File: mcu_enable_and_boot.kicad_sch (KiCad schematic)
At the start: 12 parts, among them SW1 TS_Basic_Small, SW2 TS_Basic_Small

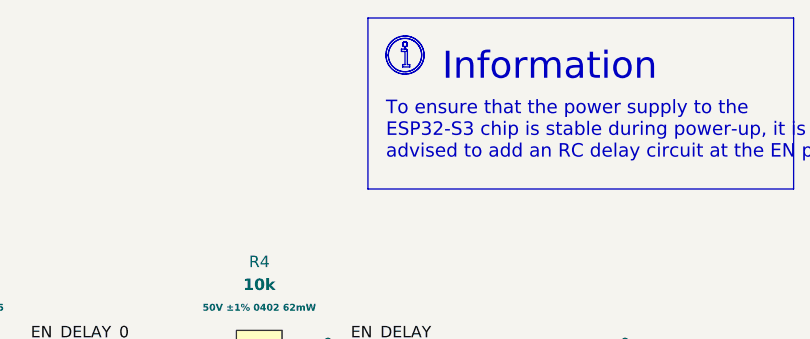
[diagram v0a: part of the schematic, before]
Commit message: Work on kibot
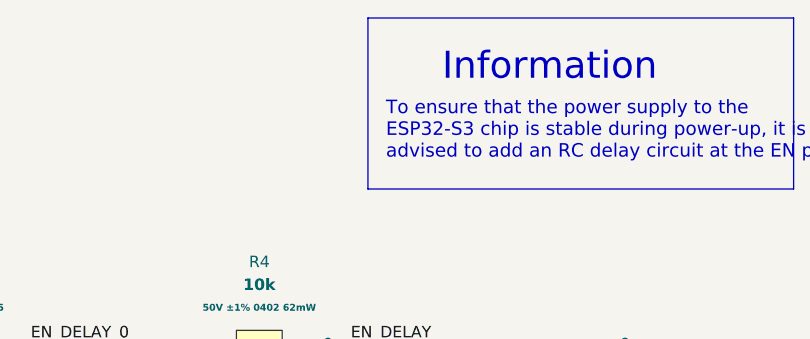
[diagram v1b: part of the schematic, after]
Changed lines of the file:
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@@
-		)
-	)
-	(polyline
-		(pts
-			(xy 127.9603 42.8818) (xy 127.9737 42.8828) (xy 127.987 42.8845) (xy 128 42.8868) (xy 128.0128 42.8898)
-			(xy 128.0253 42.8934) (xy 128.0376 42.8975) (xy 128.0497 42.9023) (xy 128.0614 42.9075) (xy 128.0728 42.9134)
-			(xy 128.0839 42.9198) (xy 128.0946 42.9266) (xy 128.105 42.934) (xy 128.115 42.9419) (xy 128.1246 42.9502)
-			(xy 128.1338 42.959) (xy 128.1425 42.9681) (xy 128.1508 42.9777) (xy 128.1587 42.9877) (xy 128.1661 42.9981)
-			(xy 128.1729 43.0088) (xy 128.1793 43.0199) (xy 128.1852 43.0313) (xy 128.1905 43.0431) (xy 128.1952 43.0551)
-			(xy 128.1994 43.0674) (xy 128.2029 43.0799) (xy 128.2059 43.0927) (xy 128.2082 43.1057) (xy 128.2099 43.119)
-			(xy 128.2109 43.1324) (xy 128.2112 43.146) (xy 128.2109 43.1597) (xy 128.2099 43.1731) (xy 128.2082 43.1863)
-			(xy 128.2059 43.1994) (xy 128.2029 43.2122) (xy 128.1994 43.2247) (xy 128.1952 43.237) (xy 128.1905 43.249)
-			(xy 128.1852 43.2607) (xy 128.1793 43.2722) (xy 128.1729 43.2832) (xy 128.1661 43.294) (xy 128.1587 43.3043)
-			(xy 128.1508 43.3143) (xy 128.1425 43.3239) (xy 128.1338 43.3331) (xy 128.1246 43.3419) (xy 128.115 43.3502)
-			(xy 128.105 43.3581) (xy 128.0946 43.3654) (xy 128.0839 43.3723) (xy 128.0728 43.3787) (xy 128.0614 43.3845)
-			(xy 128.0497 43.3898) (xy 128.0376 43.3946) (xy 128.0253 43.3987) (xy 128.0128 43.4023) (xy 128 43.4052)
-			(xy 127.987 43.4076) (xy 127.9737 43.4093) (xy 127.9603 43.4103) (xy 127.9467 43.4106) (xy 127.9331 43.4103)
-			(xy 127.9196 43.4093) (xy 127.9064 43.4076) (xy 127.8933 43.4052) (xy 127.8805 43.4023) (xy 127.868 43.3987)
-			(xy 127.8557 43.3946) (xy 127.8437 43.3898) (xy 127.832 43.3845) (xy 127.8206 43.3787) (xy 127.8095 43.3723)
-			(xy 127.7987 43.3654) (xy 127.7884 43.3581) (xy 127.7784 43.3502) (xy 127.7688 43.3419) (xy 127.7596 43.3331)
-			(xy 127.7508 43.3239) (xy 127.7425 43.3143) (xy 127.7346 43.3043) (xy 127.7273 43.294) (xy 127.7204 43.2832)
-			(xy 127.714 43.2722) (xy 127.7082 43.2607) (xy 127.7029 43.249) (xy 127.6981 43.237) (xy 127.694 43.2247)
-			(xy 127.6904 43.2122) (xy 127.6875 43.1994) (xy 127.6851 43.1863) (xy 127.6834 43.1731) (xy 127.6824 43.1597)
-			(xy 127.6821 43.146) (xy 127.6824 43.1324) (xy 127.6834 43.119) (xy 127.6851 43.1057) (xy 127.6875 43.0927)
-			(xy 127.6904 43.0799) (xy 127.694 43.0674) (xy 127.6981 43.0551) (xy 127.7029 43.0431) (xy 127.7082 43.0313)
-			(xy 127.714 43.0199) (xy 127.7204 43.0088) (xy 127.7273 42.9981) (xy 127.7346 42.9877) (xy 127.7425 42.9777)
-			(xy 127.7508 42.9681) (xy 127.7596 42.959) (xy 127.7688 42.9502) (xy 127.7784 42.9419) (xy 127.7884 42.934)
-			(xy 127.7987 42.9266) (xy 127.8095 42.9198) (xy 127.8206 42.9134) (xy 127.832 42.9075) (xy 127.8437 42.9023)
-			(xy 127.8557 42.8975) (xy 127.868 42.8934) (xy 127.8805 42.8898) (xy 127.8933 42.8868) (xy 127.9064 42.8845)
-			(xy 127.9196 42.8828) (xy 127.9331 42.8818) (xy 127.9467 42.8815) (xy 127.9603 42.8818)
-		)
-		(stroke
-			(width -0.0001)
-			(type solid)
-		)
-		(fill
-			(type color)
-			(color 34 187 51 1)
-		)
-	)
-	(polyline
-		(pts
-			(xy 127.9598 43.6755) (xy 127.9728 43.6765) (xy 127.9857 43.6781) (xy 127.9985 43.6803) (xy 128.0112 43.6832)
-			(xy 128.0236 43.6866) (xy 128.0359 43.6907) (xy 128.0479 43.6953) (xy 128.0597 43.7006) (xy 128.0713 43.7064)
-			(xy 128.0825 43.7127) (xy 128.0935 43.7197) (xy 128.1041 43.7271) (xy 128.1143 43.7351) (xy 128.1242 43.7437)
-			(xy 128.1338 43.7527) (xy 128.1428 43.7622) (xy 128.1513 43.7721) (xy 128.1593 43.7824) (xy 128.1668 43.793)
-			(xy 128.1737 43.8039) (xy 128.1801 43.8152) (xy 128.1859 43.8267) (xy 128.1911 43.8385) (xy 128.1958 43.8506)
-			(xy 128.1998 43.8628) (xy 128.2033 43.8753) (xy 128.2061 43.8879) (xy 128.2084 43.9007) (xy 128.21 43.9136)
-			(xy 128.2109 43.9267) (xy 128.2112 43.9398) (xy 128.2112 45.395) (xy 128.4758 45.395) (xy 128.4758 45.6596)
-			(xy 127.6821 45.6596) (xy 127.6821 45.395) (xy 127.9467 45.395) (xy 127.9467 43.9398) (xy 127.5498 43.9398)
-			(xy 127.5498 43.6752) (xy 127.9467 43.6752) (xy 127.9598 43.6755)
-		)
-		(stroke
-			(width -0.0001)
-			(type solid)
-		)
-		(fill
-			(type color)
-			(color 34 187 51 1)
 		)
 	)
@@
 		)
 	)
-	(polyline
-		(pts
-			(xy 128.0516 42.2226) (xy 128.1559 42.2304) (xy 128.2592 42.2432) (xy 128.3615 42.261) (xy 128.4626 42.2838)
-			(xy 128.5623 42.3115) (xy 128.6604 42.3439) (xy 128.7567 42.3811) (xy 128.8511 42.4229) (xy 128.9434 42.4694)
-			(xy 129.0334 42.5203) (xy 129.121 42.5756) (xy 129.206 42.6353) (xy 129.2881 42.6993) (xy 129.3673 42.7676)
-			(xy 129.4434 42.84) (xy 129.5158 42.916) (xy 129.584 42.9952) (xy 129.648 43.0774) (xy 129.7077 43.1623)
-			(xy 129.7631 43.2499) (xy 129.814 43.3399) (xy 129.8604 43.4323) (xy 129.9022 43.5267) (xy 129.9394 43.623)
-			(xy 129.9718 43.7211) (xy 129.9995 43.8207) (xy 130.0223 43.9218) (xy 130.0401 44.0241) (xy 130.053 44.1275)
-			(xy 130.0607 44.2317) (xy 130.0633 44.3367) (xy 130.0618 44.4167) (xy 130.0573 44.4961) (xy 130.0499 44.5749)
-			(xy 130.0396 44.6531) (xy 130.0265 44.7304) (xy 130.0105 44.807) (xy 129.9918 44.8826) (xy 129.9704 44.9573)
-			(xy 129.9463 45.031) (xy 129.9196 45.1036) (xy 129.8903 45.175) (xy 129.8584 45.2452) (xy 129.8241 45.3142)
-			(xy 129.7873 45.3818) (xy 129.7482 45.4479) (xy 129.7066 45.5126) (xy 129.6627 45.5758) (xy 129.6166 45.6373)
-			(xy 129.5682 45.6971) (xy 129.5177 45.7552) (xy 129.465 45.8115) (xy 129.4102 45.8659) (xy 129.3534 45.9184)
-			(xy 129.2945 45.9688) (xy 129.2337 46.0172) (xy 129.171 46.0634) (xy 129.1064 46.1075) (xy 129.0399 46.1492)
-			(xy 128.9717 46.1887) (xy 128.9017 46.2257) (xy 128.83 46.2602) (xy 128.7567 46.2922) (xy 128.6071 46.3477)
-			(xy 128.4553 46.3914) (xy 128.302 46.4234) (xy 128.1477 46.4439) (xy 127.9931 46.4529) (xy 127.8389 46.4506)
-			(xy 127.6855 46.4372) (xy 127.5337 46.4127) (xy 127.3841 46.3772) (xy 127.2373 46.331) (xy 127.0939 46.274)
-			(xy 126.9545 46.2065) (xy 126.8198 46.1286) (xy 126.6904 46.0403) (xy 126.5669 45.9419) (xy 126.45 45.8334)
-			(xy 126.3414 45.7164) (xy 126.243 45.5929) (xy 126.1547 45.4635) (xy 126.0768 45.3288) (xy 126.0093 45.1894)
-			(xy 125.9524 45.046) (xy 125.9061 44.8992) (xy 125.8707 44.7496) (xy 125.8462 44.5978) (xy 125.8327 44.4445)
-			(xy 125.8317 44.3773) (xy 126.095 44.3773) (xy 126.1029 44.5126) (xy 126.1208 44.6476) (xy 126.1488 44.7817)
-			(xy 126.187 44.9145) (xy 126.2356 45.0454) (xy 126.2938 45.1723) (xy 126.3607 45.2933) (xy 126.4357 45.4079)
-			(xy 126.5185 45.516) (xy 126.6086 45.6173) (xy 126.7054 45.7113) (xy 126.8086 45.7979) (xy 126.9177 45.8766)
-			(xy 127.0322 45.9473) (xy 127.1517 46.0095) (xy 127.2756 46.063) (xy 127.4036 46.1074) (xy 127.5352 46.1425)
-			(xy 127.6698 46.168) (xy 127.8072 46.1835) (xy 127.9467 46.1887) (xy 128.0385 46.1865) (xy 128.1297 46.1797)
-			(xy 128.2202 46.1685) (xy 128.3097 46.1528) (xy 128.3981 46.1329) (xy 128.4853 46.1087) (xy 128.5711 46.0803)
-			(xy 128.6554 46.0478) (xy 128.738 46.0112) (xy 128.8188 45.9706) (xy 128.8976 45.926) (xy 128.9742 45.8776)
-			(xy 129.0485 45.8253) (xy 129.1204 45.7693) (xy 129.1897 45.7096) (xy 129.2563 45.6463) (xy 129.3196 45.5797)
-			(xy 129.3793 45.5104) (xy 129.4353 45.4385) (xy 129.4876 45.3642) (xy 129.536 45.2876) (xy 129.5806 45.2088)
-			(xy 129.6212 45.128) (xy 129.6578 45.0454) (xy 129.6903 44.9611) (xy 129.7187 44.8753) (xy 129.7429 44.7881)
-			(xy 129.7628 44.6997) (xy 129.7785 44.6102) (xy 129.7897 44.5197) (xy 129.7965 44.4285) (xy 129.7987 44.3367)
-			(xy 129.7974 44.2667) (xy 129.7935 44.1972) (xy 129.787 44.1282) (xy 129.778 44.0598) (xy 129.7665 43.9921)
-			(xy 129.7525 43.9252) (xy 129.7362 43.859) (xy 129.7174 43.7936) (xy 129.6963 43.7291) (xy 129.673 43.6656)
-			(xy 129.6473 43.6031) (xy 129.6195 43.5417) (xy 129.5894 43.4813) (xy 129.5573 43.4222) (xy 129.523 43.3643)
-			(xy 129.4866 43.3077) (xy 129.4482 43.2525) (xy 129.4079 43.1986) (xy 129.3655 43.1463) (xy 129.3213 43.0954)
-			(xy 129.2752 43.0462) (xy 129.2273 42.9986) (xy 129.1775 42.9527) (xy 129.126 42.9085) (xy 129.0728 42.8662)
-			(xy 129.0179 42.8257) (xy 128.9614 42.7872) (xy 128.9033 42.7507) (xy 128.8436 42.7162) (xy 128.7823 42.6838)
-			(xy 128.7196 42.6536) (xy 128.6554 42.6256) (xy 128.5245 42.577) (xy 128.3917 42.5388) (xy 128.2576 42.5108)
-			(xy 128.1226 42.4929) (xy 127.9873 42.485) (xy 127.8523 42.487) (xy 127.7182 42.4987) (xy 127.5853 42.5202)
-			(xy 127.4544 42.5512) (xy 127.326 42.5917) (xy 127.2005 42.6415) (xy 127.0786 42.7005) (xy 126.9607 42.7687)
-			(xy 126.8475 42.846) (xy 126.7394 42.9321) (xy 126.637 43.027) (xy 126.5421 43.1294) (xy 126.456 43.2375)
-			(xy 126.3787 43.3507) (xy 126.3105 43.4686) (xy 126.2515 43.5905) (xy 126.2017 43.716) (xy 126.1612 43.8444)
-			(xy 126.1302 43.9753) (xy 126.1087 44.1082) (xy 126.097 44.2423) (xy 126.095 44.3773) (xy 125.8317 44.3773)
-			(xy 125.8304 44.2902) (xy 125.8395 44.1356) (xy 125.8599 43.9814) (xy 125.8919 43.828) (xy 125.9356 43.6763)
-			(xy 125.9911 43.5267) (xy 126.0577 43.3816) (xy 126.1341 43.2434) (xy 126.2199 43.1124) (xy 126.3145 42.9888)
-			(xy 126.4174 42.8731) (xy 126.5281 42.7656) (xy 126.646 42.6667) (xy 126.7707 42.5767) (xy 126.9016 42.496)
-			(xy 127.0381 42.4249) (xy 127.1797 42.3637) (xy 127.326 42.3129) (xy 127.4764 42.2728) (xy 127.6303 42.2437)
-			(xy 127.7872 42.226) (xy 127.9467 42.22) (xy 128.0516 42.2226)
-		)
-		(stroke
-			(width -0.0001)
-			(type solid)
-		)
-		(fill
-			(type color)
-			(color 34 187 51 1)
-		)
-	)
